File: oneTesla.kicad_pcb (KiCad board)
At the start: 2 copper layers, 100 x 100 mm, 45 parts, among them IC1 74HCT14, IC2 74HCT74, IC3 UCC37321P, IC4 UCC37321P, IC6 MC7805BDTRKG, J1 2EDGRC-5.08-02P, J110 Jumper 110V, P1 PRIMARIO A, P2 PRIMARIO B, Q1 FGA60N65SMD, Q2 FGA60N65SMD, T1 1:1:1, T3 1:300

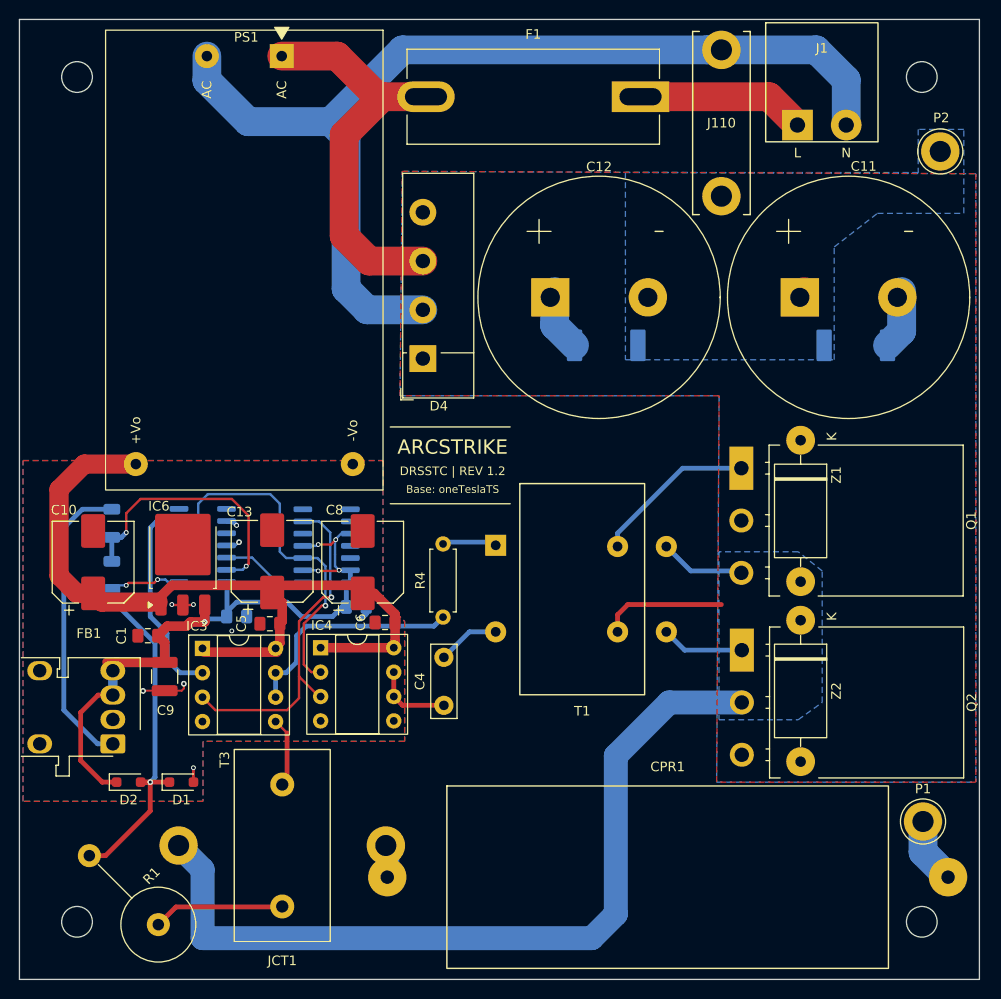
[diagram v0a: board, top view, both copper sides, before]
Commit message: chore: save latest PCB routing and silkscreen edits
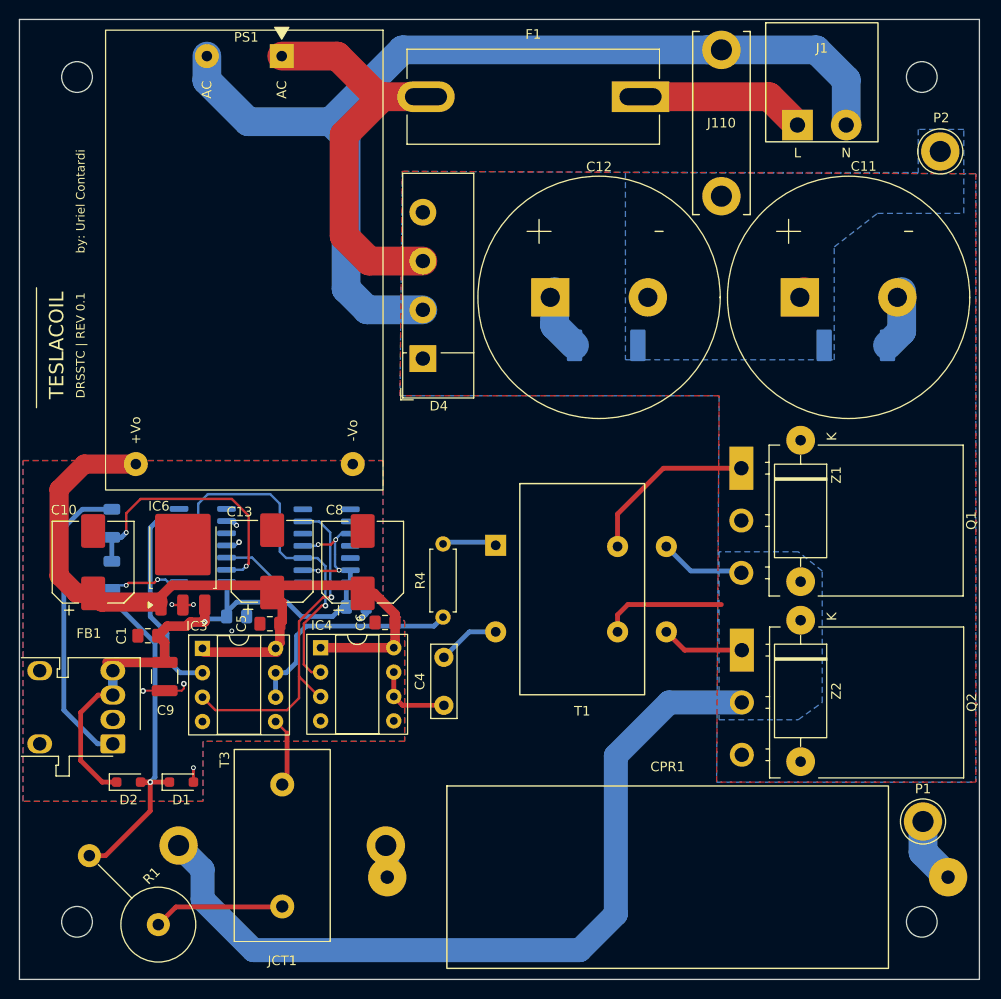
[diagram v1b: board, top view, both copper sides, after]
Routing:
- net /SW_NODE: track 95.6 -> 94.3 mm
- net /GATE_H: track 17.1 -> 18.3 mm
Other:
- board text added: "DRSSTC | REV 0.1"
- board text added: "TESLACOIL"
- board text added: "by: Uriel Contardi"
- board text removed: "ARCSTRIKE"
- board text removed: "Base: oneTeslaTS"
- board text removed: "DRSSTC | REV 1.2"
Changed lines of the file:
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@@
 	)
 	(gr_line
-		(start 70 69.5)
-		(end 82.5 69.5)
-		(stroke
-			(width 0.12)
-			(type solid)
-		)
-		(layer "F.SilkS")
-	)
-	(gr_line
-		(start 70 77.5)
-		(end 82.5 77.5)
+		(start 33.15 67.5)
+		(end 33.15 55)
 		(stroke
 			(width 0.12)
@@
 		)
 	)
-	(gr_text "Base: oneTeslaTS"
-		(at 76.5 76 0)
+	(gr_text "by: Uriel Contardi\n"
+		(at 37.75 46 90)
 		(layer "F.SilkS")
 		(effects
 			(font
-				(size 0.8 0.8)
-				(thickness 0.12)
+				(size 0.9 0.9)
+				(thickness 0.15)
 			)
 		)
 	)
-	(gr_text "DRSSTC | REV 1.2"
-		(at 76.5 74.1 0)
+	(gr_text "DRSSTC | REV 0.1"
+		(at 37.75 61 90)
 		(layer "F.SilkS")
 		(effects
@@
 		)
 	)
-	(gr_text "ARCSTRIKE"
-		(at 76.5 71.6 0)
+	(gr_text "TESLACOIL"
+		(at 35.25 61 90)
 		(layer "F.SilkS")
 		(effects
@@
 	)
 	(segment
-		(start 100.668 92.75)
-		(end 106.625 92.75)
-		(width 0.5)
-		(layer "B.Cu")
-		(net "/GATE_L")
-	)
-	(segment
 		(start 98.763 90.845)
 		(end 100.668 92.75)
 		(width 0.5)
-		(layer "B.Cu")
+		(layer "F.Cu")
 		(net "/GATE_L")
 	)
 	(segment
-		(start 93.5 103.75)
-		(end 93.5 120.25)
-		(width 2.5)
-		(layer "B.Cu")
-		(net "/SW_NODE")
+		(start 100.668 92.75)
+		(end 106.625 92.75)
+		(width 0.5)
+		(layer "F.Cu")
+		(net "/GATE_L")
 	)
 	(segment
-		(start 50.455 122.75)
-		(end 50.455 115.6)
+		(start 50.455 115.6)
+		(end 47.955 113.1)
 		(width 2.5)
 		(layer "B.Cu")
@@
 	)
 	(segment
-		(start 93.5 120.25)
-		(end 91 122.75)
+		(start 89.75 124)
+		(end 55.75 124)
 		(width 2.5)
 		(layer "B.Cu")
@@
 	)
 	(segment
-		(start 50.455 115.6)
-		(end 47.955 113.1)
+		(start 50.455 118.705)
+		(end 50.455 115.6)
 		(width 2.5)
 		(layer "B.Cu")
@@
 	)
 	(segment
-		(start 91 122.75)
-		(end 50.455 122.75)
+		(start 93.5 103.75)
+		(end 93.5 120.25)
+		(width 2.5)
+		(layer "B.Cu")
+		(net "/SW_NODE")
+	)
+	(segment
+		(start 93.5 120.25)
+		(end 89.75 124)
 		(width 2.5)
 		(layer "B.Cu")
@@
 	)
 	(segment
+		(start 55.75 124)
+		(end 50.455 118.705)
+		(width 2.5)
+		(layer "B.Cu")
+		(net "/SW_NODE")
+	)
+	(segment
 		(start 106.775 103.5)
 		(end 106.625 103.65)
@@
 	)
 	(segment
-		(start 100.45 73.8)
+		(start 98.45 73.8)
 		(end 106.575 73.8)
 		(width 0.5)
-		(layer "B.Cu")
+		(layer "F.Cu")
 		(net "/GATE_H")
 	)
 	(segment
-		(start 93.683 81.955)
-		(end 93.683 80.567)
+		(start 93.683 78.567)
+		(end 98.45 73.8)
 		(width 0.5)
-		(layer "B.Cu")
+		(layer "F.Cu")
 		(net "/GATE_H")
 	)
 	(segment
-		(start 93.683 80.567)
-		(end 100.45 73.8)
+		(start 93.683 81.955)
+		(end 93.683 78.567)
 		(width 0.5)
-		(layer "B.Cu")
+		(layer "F.Cu")
 		(net "/GATE_H")
 	)
